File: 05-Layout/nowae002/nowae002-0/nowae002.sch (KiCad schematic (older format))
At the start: 56 parts, among them J1 SMALL_JUMPER, J2 SMALL_JUMPER, P1 USB_A_90, Q1 IRLML6402, U1 FT230XQ, U2 TPS62152, U3 RN4870

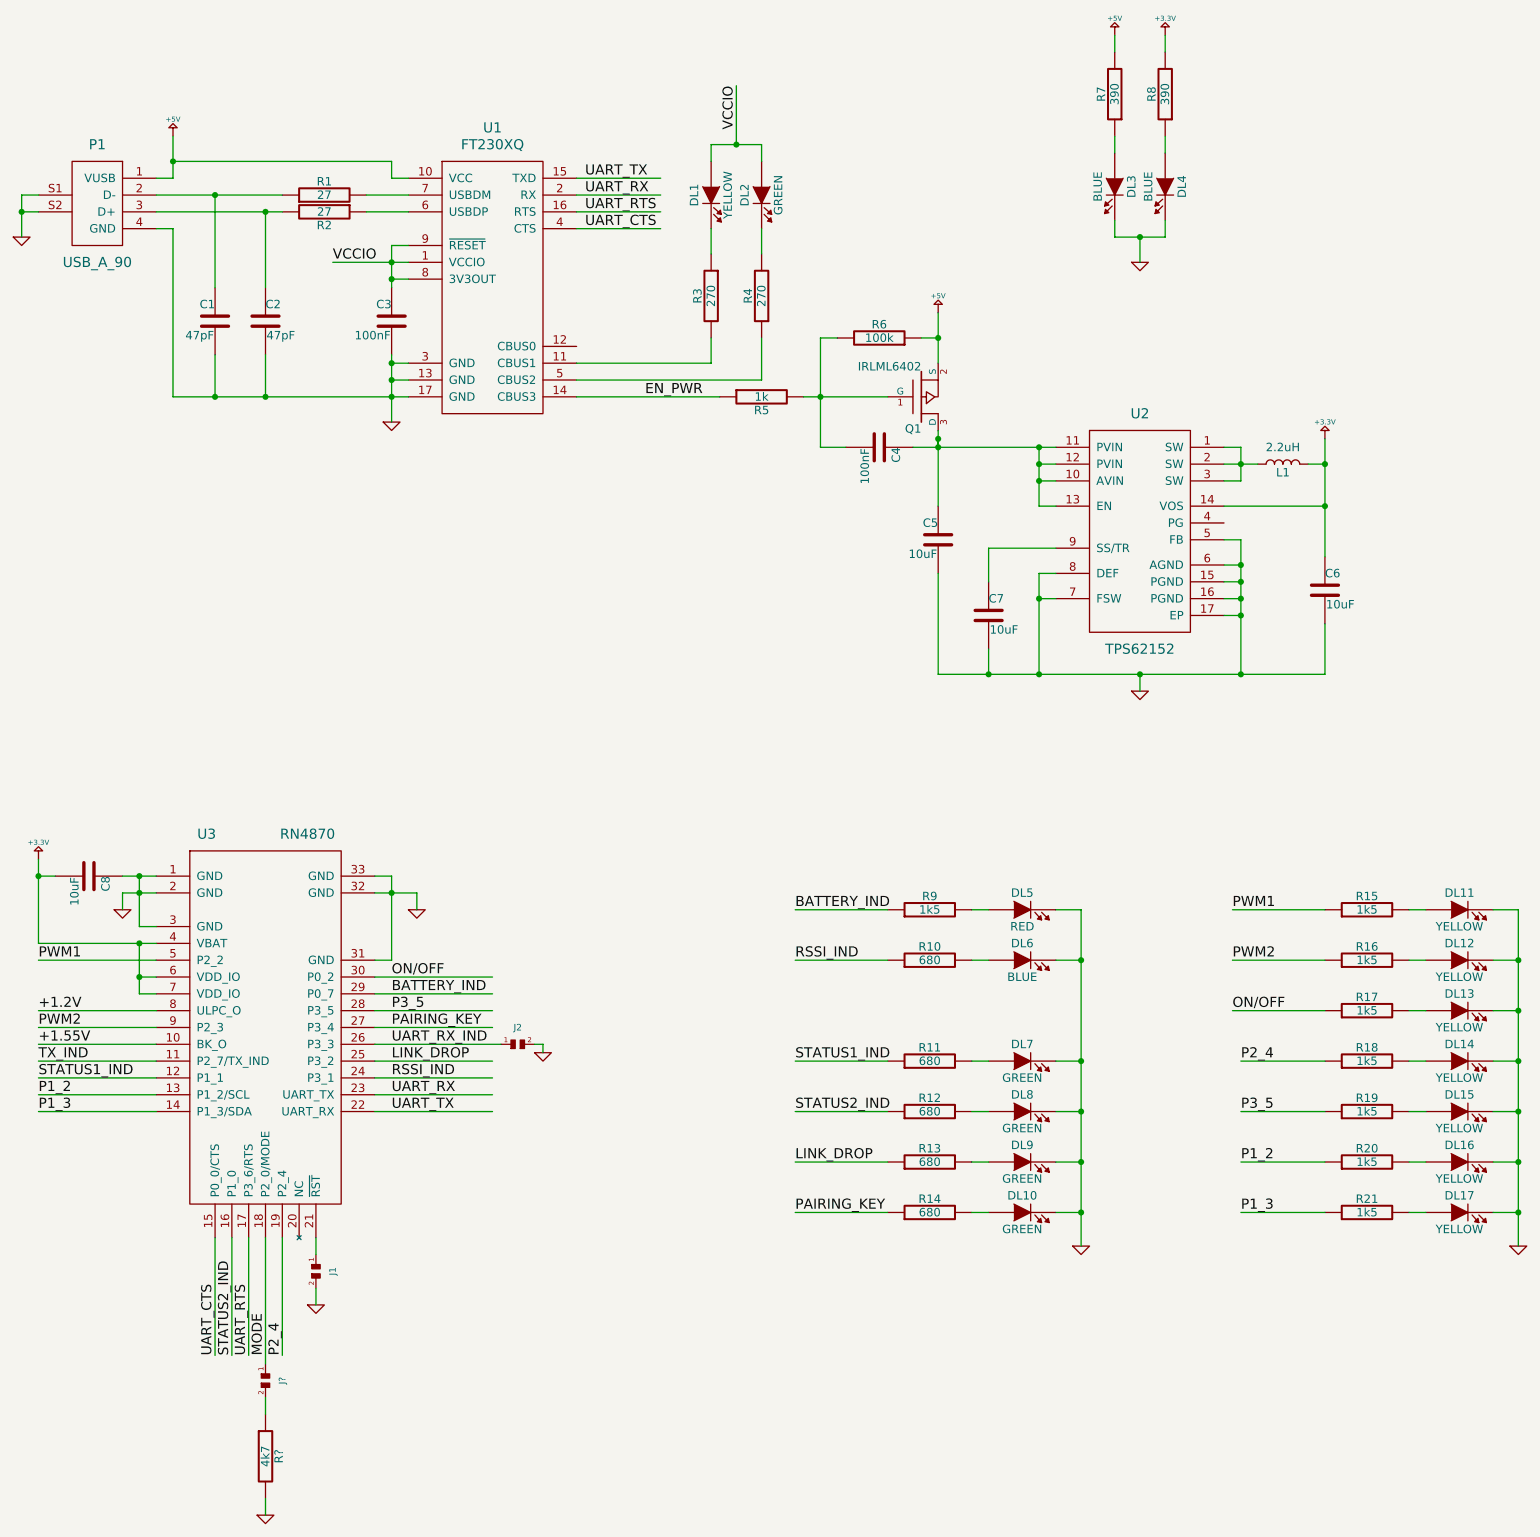
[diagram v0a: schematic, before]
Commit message: Minor fixes (nowae002)
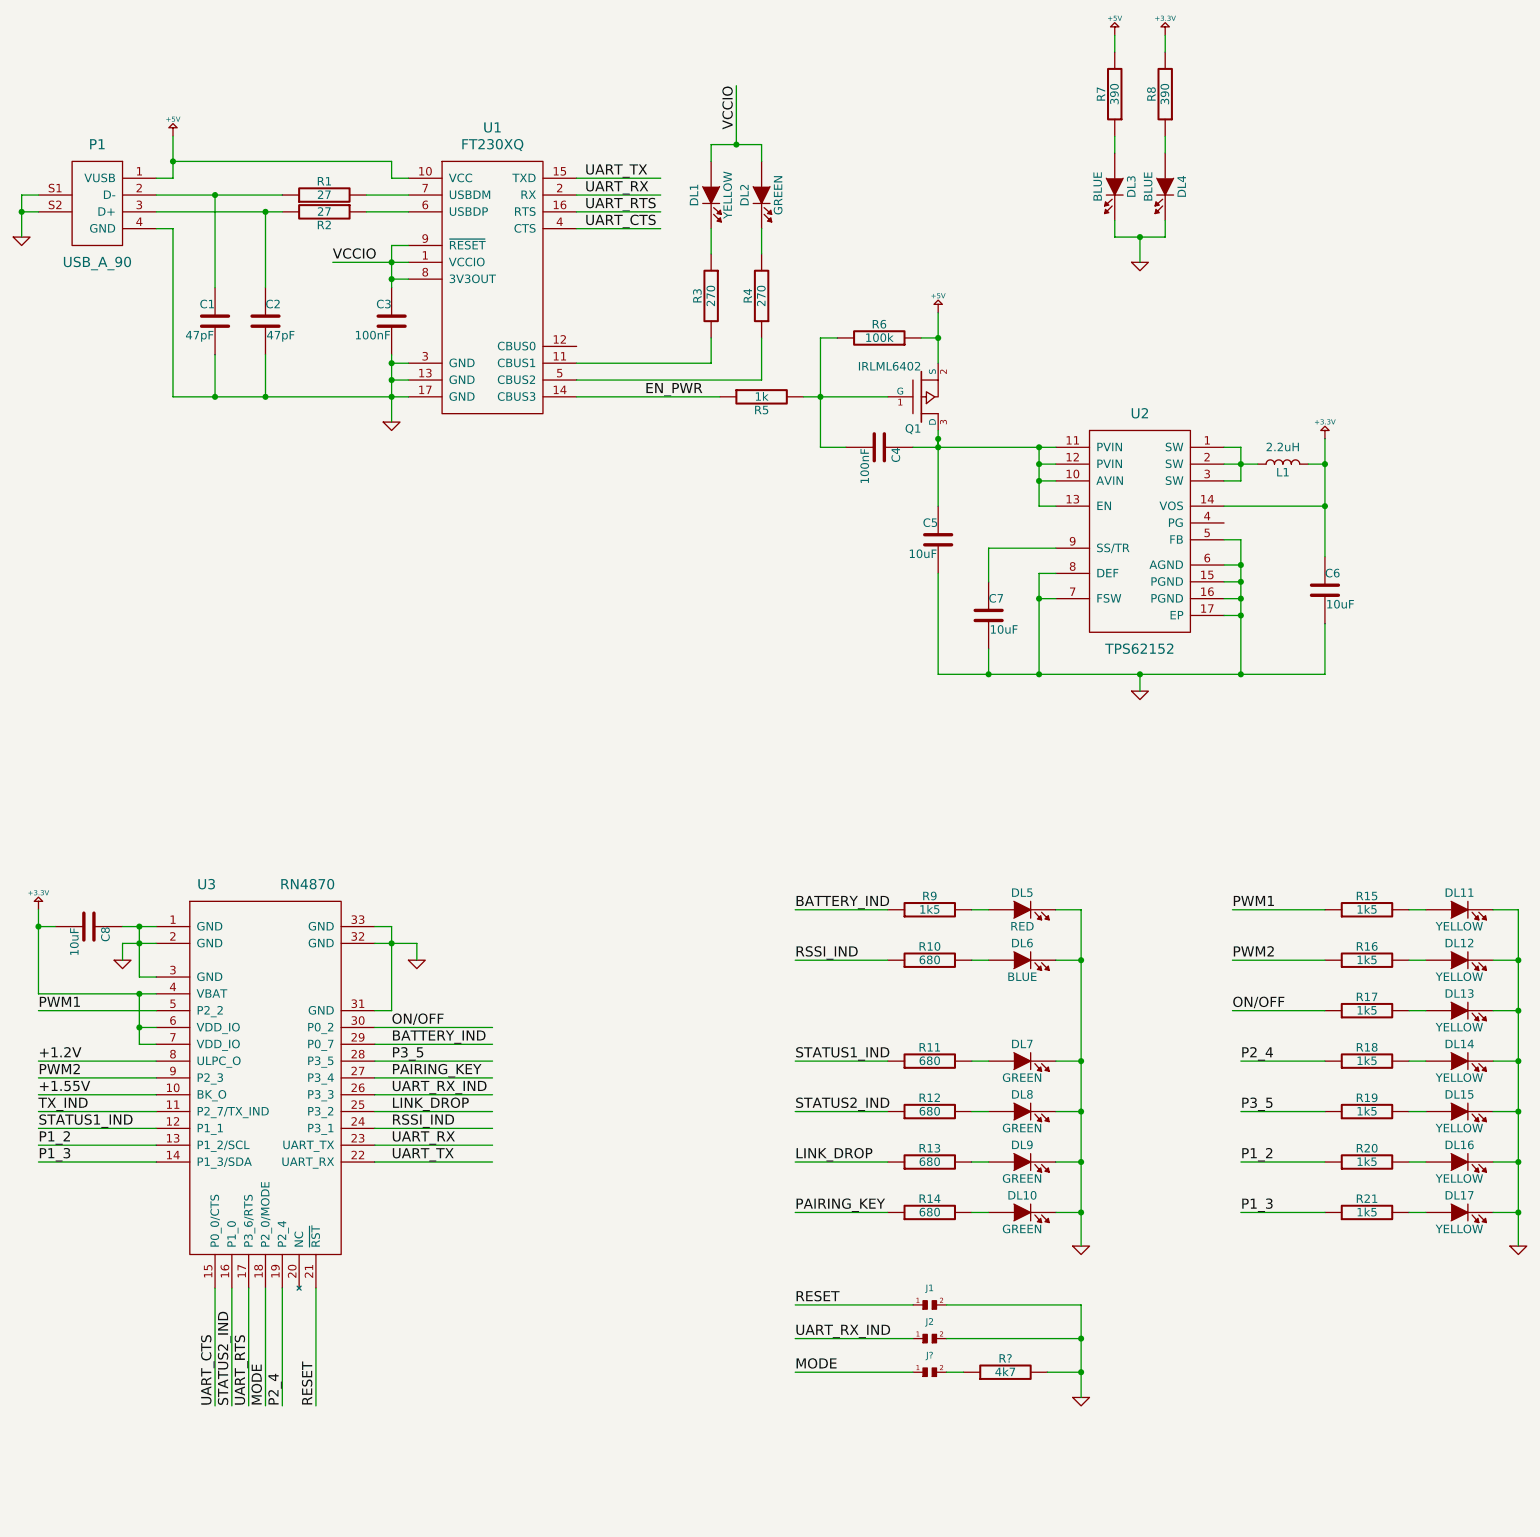
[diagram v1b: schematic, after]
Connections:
- net labels added: RESET
- wire segments 170 -> 231
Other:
- moved on the sheet: C8, J1, J2, J?, R?, U3
